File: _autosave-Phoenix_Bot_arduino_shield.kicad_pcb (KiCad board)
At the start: 2 copper layers, 135.9 x 64.8 mm, 46 parts, among them J1 Analog_signal_male, J10 Ground, J11 Ground, J12 Ground, J13 12V_terminal, J14 PWN(10-5), J15 On Board Supply, J16 1x8 Male, J17 1x8 Male, J18 PWM_(6-1), J19 Analog_Pin_1, J2 Encoder_signal, J20 1x8 Female, J21 1x8 Female, J22 Serial, J23 ICSP, J24 Analog_Pin_2, J25 Digital_Pins, J27 Solenoid_terminal, J28 Solendoid_middle_terminal, J29 bottom_solenoid_terminal, J3 Servo_signal, J4 Analog_signal_female, J5 Analog_signal_power, J6 Servo_Power, J7 Encoder_Power, J8 Analog_Power_female, J9 Ground, q1 solenoid_1, q2 solenoid_4, q3 solenoid_3, q4 solenoid_5, q5 solenoid_3, q6 solenoid_6

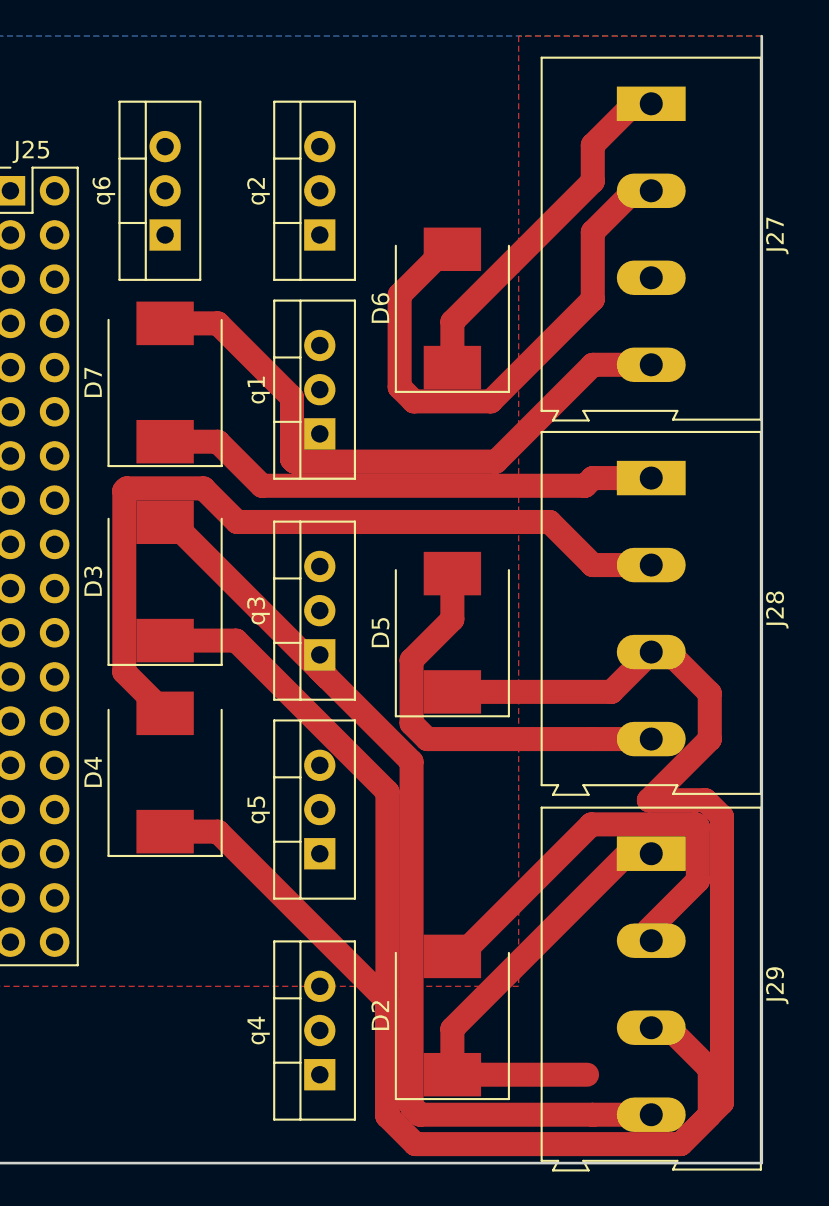
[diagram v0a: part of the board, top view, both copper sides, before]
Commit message: Began board layout
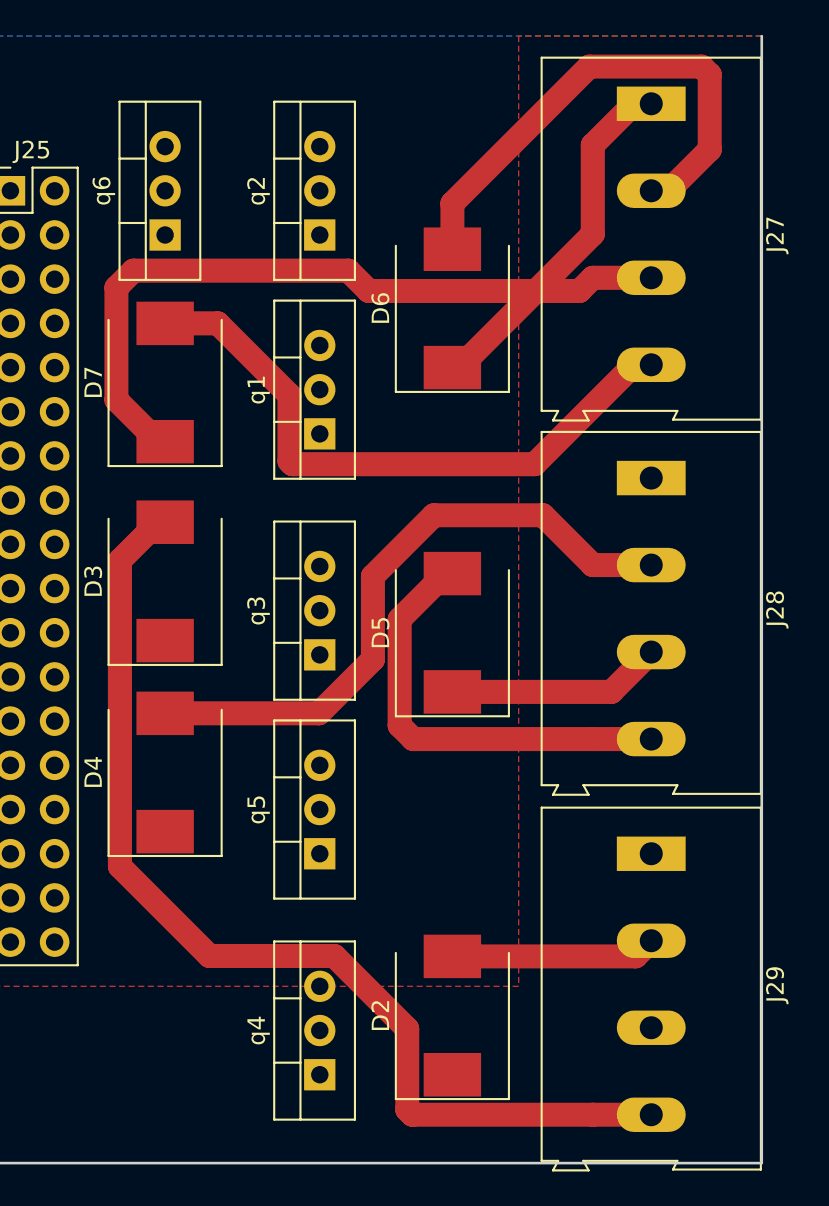
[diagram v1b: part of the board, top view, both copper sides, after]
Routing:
- net +12V: track 210.6 -> 75.3 mm
- net /Drain_1: track 26.3 -> 11.8 mm
- net /Drain_3: track 46.0 -> 36.6 mm
- net /Drain_2: track 55.1 -> 60.3 mm
- net /Drain_5: track 31.5 -> 29.5 mm
- net /Drain_4: track 23.7 -> 25.0 mm
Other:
- net class Default: clearance 0.006 -> 0.1524; trace_width 0.006 -> 0.1524; via_dia 0.027 -> 0.6858; via_drill 0.013 -> 0.3302
- net class Powertrace: clearance 0.006 -> 0.254; trace_width 0.0544 -> 1.38176; via_dia 0.027 -> 0.6858; via_drill 0.013 -> 0.3302
- rule trace_clearance: 0.006 -> 0.1524
- rule trace_min: 0.006 -> 0.1524
- rule via_min_drill: 0.013 -> 0.3302
- rule via_min_size: 0.027 -> 0.6858
